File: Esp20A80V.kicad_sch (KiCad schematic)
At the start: 20 parts, among them J1 dcdc, J2 free, J4 I2C/Uart, Q1 SI2305, SW1 3x button, U1 spi tft with touch (+ sd card), U3 20A 80V dcdc, U4 Wemos S2 Mini

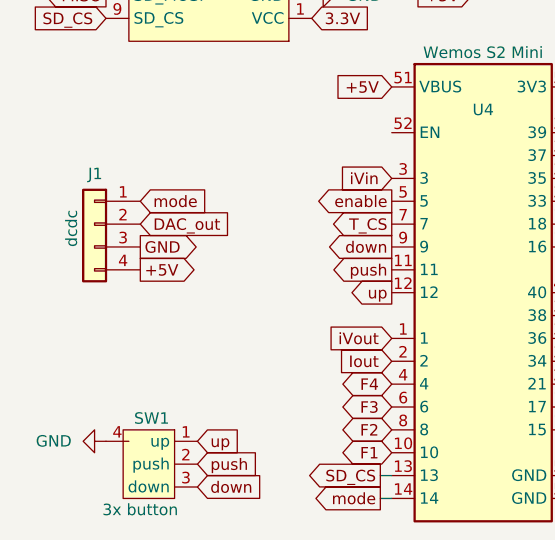
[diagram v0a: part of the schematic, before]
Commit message: update
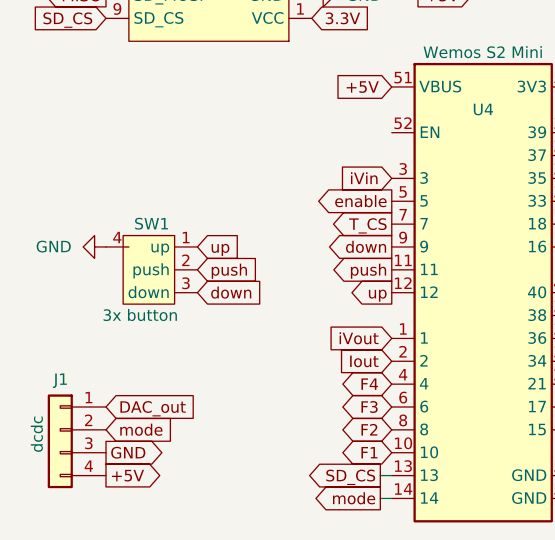
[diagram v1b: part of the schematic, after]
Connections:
- net DAC_out: now also J1.1 (Pin_1); no longer J1.2 (Pin_2)
- net mode: now also J1.2 (Pin_2); no longer J1.1 (Pin_1)
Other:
- moved on the sheet: J1, SW1
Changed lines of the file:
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@@
     )
   )
-  (global_label "push" (shape input) (at 107.95 118.11 0) (fields_autoplaced)
-    (effects (font (size 1.27 1.27)) (justify left))
-    (property "Intersheetrefs" "${INTERSHEET_REFS}" (at 115.4103 118.11 0)
+  (global_label "push" (shape input) (at 107.95 96.52 0) (fields_autoplaced)
+    (effects (font (size 1.27 1.27)) (justify left))
+    (property "Intersheetrefs" "${INTERSHEET_REFS}" (at 115.4103 96.52 0)
       (effects (font (size 1.27 1.27)) (justify left) hide)
     )
@@
     )
   )
-  (global_label "up" (shape input) (at 107.95 115.57 0) (fields_autoplaced)
-    (effects (font (size 1.27 1.27)) (justify left))
-    (property "Intersheetrefs" "${INTERSHEET_REFS}" (at 113.2332 115.57 0)
+  (global_label "up" (shape input) (at 107.95 93.98 0) (fields_autoplaced)
+    (effects (font (size 1.27 1.27)) (justify left))
+    (property "Intersheetrefs" "${INTERSHEET_REFS}" (at 113.2332 93.98 0)
       (effects (font (size 1.27 1.27)) (justify left) hide)
     )
@@
     )
   )
-  (global_label "DAC_out" (shape input) (at 101.6 91.44 0) (fields_autoplaced)
-    (effects (font (size 1.27 1.27)) (justify left))
-    (property "Intersheetrefs" "${INTERSHEET_REFS}" (at 112.2051 91.44 0)
-      (effects (font (size 1.27 1.27)) (justify left) hide)
-    )
-  )
-  (global_label "GND" (shape output) (at 101.6 93.98 0) (fields_autoplaced)
-    (effects (font (size 1.27 1.27)) (justify left))
-    (property "Intersheetrefs" "${INTERSHEET_REFS}" (at 108.4557 93.98 0)
+  (global_label "DAC_out" (shape input) (at 97.79 111.76 0) (fields_autoplaced)
+    (effects (font (size 1.27 1.27)) (justify left))
+    (property "Intersheetrefs" "${INTERSHEET_REFS}" (at 108.3951 111.76 0)
+      (effects (font (size 1.27 1.27)) (justify left) hide)
+    )
+  )
+  (global_label "GND" (shape output) (at 97.79 116.84 0) (fields_autoplaced)
+    (effects (font (size 1.27 1.27)) (justify left))
+    (property "Intersheetrefs" "${INTERSHEET_REFS}" (at 104.6457 116.84 0)
       (effects (font (size 1.27 1.27)) (justify left) hide)
     )
@@
     )
   )
-  (global_label "+5V" (shape output) (at 101.6 96.52 0) (fields_autoplaced)
-    (effects (font (size 1.27 1.27)) (justify left))
-    (property "Intersheetrefs" "${INTERSHEET_REFS}" (at 108.4557 96.52 0)
+  (global_label "+5V" (shape output) (at 97.79 119.38 0) (fields_autoplaced)
+    (effects (font (size 1.27 1.27)) (justify left))
+    (property "Intersheetrefs" "${INTERSHEET_REFS}" (at 104.6457 119.38 0)
       (effects (font (size 1.27 1.27)) (justify left) hide)
     )
@@
     )
   )
-  (global_label "down" (shape input) (at 107.95 120.65 0) (fields_autoplaced)
-    (effects (font (size 1.27 1.27)) (justify left))
-    (property "Intersheetrefs" "${INTERSHEET_REFS}" (at 115.7127 120.65 0)
+  (global_label "down" (shape input) (at 107.95 99.06 0) (fields_autoplaced)
+    (effects (font (size 1.27 1.27)) (justify left))
+    (property "Intersheetrefs" "${INTERSHEET_REFS}" (at 115.7127 99.06 0)
       (effects (font (size 1.27 1.27)) (justify left) hide)
     )
@@
     )
   )
-  (global_label "mode" (shape input) (at 101.6 88.9 0) (fields_autoplaced)
-    (effects (font (size 1.27 1.27)) (justify left))
-    (property "Intersheetrefs" "${INTERSHEET_REFS}" (at 109.6651 88.9 0)
+  (global_label "mode" (shape input) (at 97.79 114.3 0) (fields_autoplaced)
+    (effects (font (size 1.27 1.27)) (justify left))
+    (property "Intersheetrefs" "${INTERSHEET_REFS}" (at 105.8551 114.3 0)
       (effects (font (size 1.27 1.27)) (justify left) hide)
     )
@@
     )
   )
-  (symbol (lib_id "Connector_Generic:Conn_01x04") (at 96.52 91.44 0) (mirror y) (unit 1)
-    (in_bom yes) (on_board yes) (dnp no)
-    (property "Reference" "J1" (at 97.409 85.852 0)
-      (effects (font (size 1.27 1.27)) (justify left))
-    )
-    (property "Value" "dcdc" (at 93.98 93.98 90)
-      (effects (font (size 1.27 1.27)) (justify left))
-    )
-    (property "Footprint" "Connector_JST:JST_PH_B4B-PH-K_1x04_P2.00mm_Vertical" (at 93.98 91.44 90)
-      (effects (font (size 1.27 1.27)) hide)
-    )
-    (property "Datasheet" "~" (at 96.52 91.44 0)
+  (symbol (lib_id "Connector_Generic:Conn_01x04") (at 92.71 114.3 0) (mirror y) (unit 1)
+    (in_bom yes) (on_board yes) (dnp no)
+    (property "Reference" "J1" (at 93.599 108.712 0)
+      (effects (font (size 1.27 1.27)) (justify left))
+    )
+    (property "Value" "dcdc" (at 90.17 116.84 90)
+      (effects (font (size 1.27 1.27)) (justify left))
+    )
+    (property "Footprint" "Connector_JST:JST_PH_B4B-PH-K_1x04_P2.00mm_Vertical" (at 90.17 114.3 90)
+      (effects (font (size 1.27 1.27)) hide)
+    )
+    (property "Datasheet" "~" (at 92.71 114.3 0)
       (effects (font (size 1.27 1.27)) hide)
     )
@@
     )
   )
-  (symbol (lib_id "Esp20A80V:3way_dial_switch") (at 105.41 120.65 0) (mirror y) (unit 1)
-    (in_bom yes) (on_board yes) (dnp no)
-    (property "Reference" "SW1" (at 102.87 113.03 0)
-      (effects (font (size 1.27 1.27)))
-    )
-    (property "Value" "3x button" (at 101.6 123.19 0)
-      (effects (font (size 1.27 1.27)))
-    )
-    (property "Footprint" "Esp20A80V:3way dial switch" (at 102.87 125.095 0)
-      (effects (font (size 1.27 1.27)) hide)
-    )
-    (property "Datasheet" "" (at 107.95 118.11 90)
+  (symbol (lib_id "Esp20A80V:3way_dial_switch") (at 105.41 99.06 0) (mirror y) (unit 1)
+    (in_bom yes) (on_board yes) (dnp no)
+    (property "Reference" "SW1" (at 102.87 91.44 0)
+      (effects (font (size 1.27 1.27)))
+    )
+    (property "Value" "3x button" (at 101.6 101.6 0)
+      (effects (font (size 1.27 1.27)))
+    )
+    (property "Footprint" "Esp20A80V:3way dial switch" (at 102.87 103.505 0)
+      (effects (font (size 1.27 1.27)) hide)
+    )
+    (property "Datasheet" "" (at 107.95 96.52 90)
       (effects (font (size 1.27 1.27)) hide)
     )
@@
     )
   )
-  (symbol (lib_id "power:GND") (at 97.79 115.57 270) (unit 1)
+  (symbol (lib_id "power:GND") (at 97.79 93.98 270) (unit 1)
     (in_bom yes) (on_board yes) (dnp no) (fields_autoplaced)
-    (property "Reference" "#PWR01" (at 91.44 115.57 0)
-      (effects (font (size 1.27 1.27)) hide)
-    )
-    (property "Value" "GND" (at 93.98 115.57 90)
-      (effects (font (size 1.27 1.27)) (justify right))
-    )
-    (property "Footprint" "" (at 97.79 115.57 0)
-      (effects (font (size 1.27 1.27)) hide)
-    )
-    (property "Datasheet" "" (at 97.79 115.57 0)
-      (effects (font (size 1.27 1.27)) hide)
-    )
+    (property "Reference" "#PWR01" (at 91.44 93.98 0)
+      (effects (font (size 1.27 1.27)) hide)
+    )
+    (property "Value" "GND" (at 93.98 93.98 90)
+      (effects (font (size 1.27 1.27)) (justify right))
+    )
+    (property "Footprint" "" (at 97.79 93.98 0)
+      (effects (font (size 1.27 1.27)) hide)
+    )
+    (property "Datasheet" "" (at 97.79 93.98 0)
+      (effects (font (size 1.27 1.27)) hide)
+    )
